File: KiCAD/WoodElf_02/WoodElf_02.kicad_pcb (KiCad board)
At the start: 2 copper layers, 19.2 x 19.2 mm, 20 parts

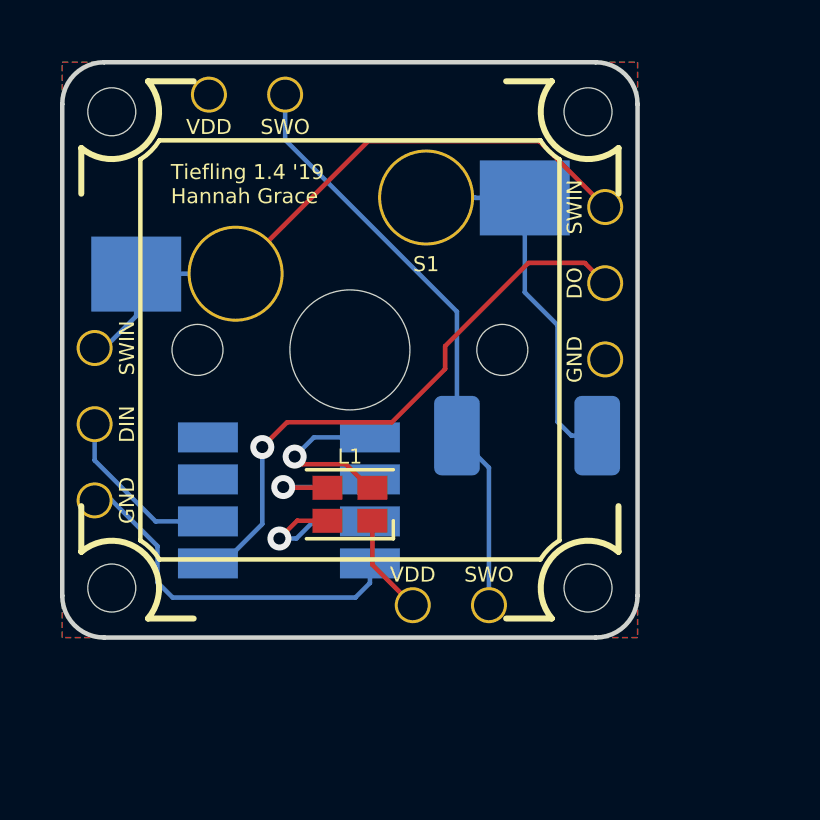
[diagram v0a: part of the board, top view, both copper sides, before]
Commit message: Added a logo
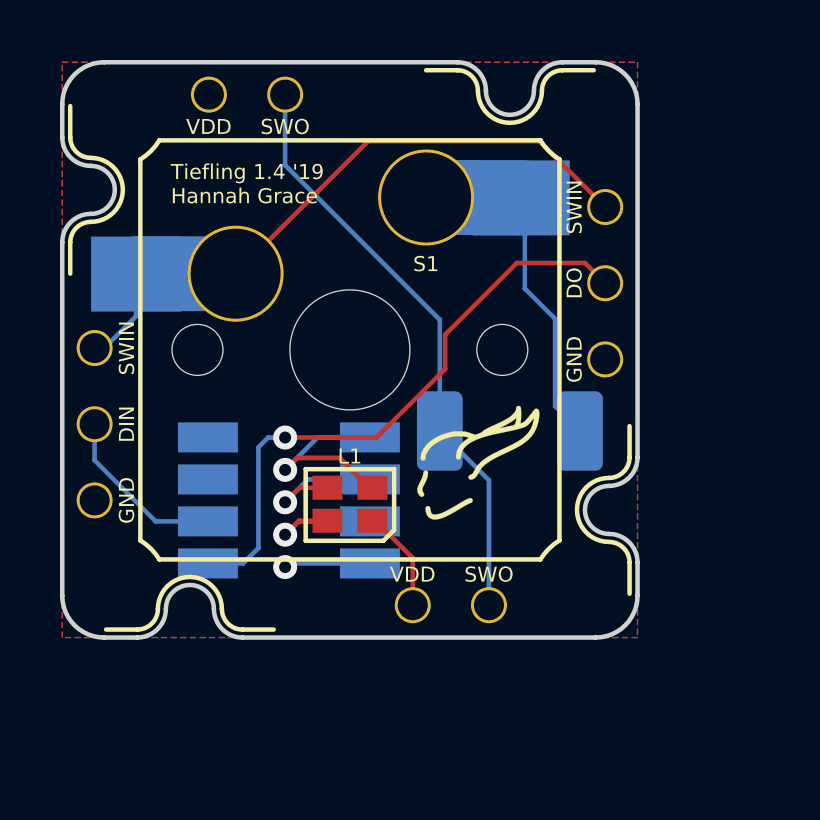
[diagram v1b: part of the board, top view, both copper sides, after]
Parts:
- removed the Mount at (148.6, 99.7)
- removed the Mount at (132.7, 99.7)
- added G***: Tiefling_Logo, WoodElf_Lib:Tiefling_Logo, F.Cu at (144.9, 111.6)
- added G***: Tiefling_LogoSmall, WoodElf_Lib:Tiefling_LogoSmall, B.Cu at (148.3, 115.4)
- added Mount: Mount, WoodElf_Lib:Mount, F.Cu at (146.0, 99.0)
- added Mount: Mount, WoodElf_Lib:Mount, F.Cu at (132.0, 102.3)
- moved Mount 2.70 mm to (135.3, 116.3), turned to 180 degrees
- moved Mount 2.70 mm to (149.3, 113.0), turned to 270 degrees
- moved D1 0.59 mm to (146.0, 110.3)
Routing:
- net /GND: track 12.1 -> 2.88 mm, vias 0 -> 1
- net Net-(C1-Pad3): track 6.48 -> 5.11 mm
- net Net-(D1-Pad1): track 13.5 -> 12.6 mm
- net /DO: track 19.6 -> 20.3 mm
- net Net-(C1-Pad2): track 4.48 -> 5.12 mm
- net Net-(C1-Pad1): track 6.16 -> 6.76 mm
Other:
- outline, holes or cut-outs redrawn
- board text added: "Tiefling Hannah Grace 1.4 '19"
